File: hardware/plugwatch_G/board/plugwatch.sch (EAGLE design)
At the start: 176 parts, among them J1 DM3AT-SF-PEJM5, J2 SCREW_TERMNIAL_1, J3 SCREW_TERMNIAL_1, J4 TC2030-JLINK-L, Q1 NX3008PBK, Q2 MOSFET-NCHANNELSMD, U1 AB1815-T3, U10 STM32L432KC, U11 SIP32510, U12 SIP32510, U13 ADA4096-4ACPZ-R7, U14 SIP32510, U15 REF2030AIDDCR, U16 TCA9406DCUR, U17 SN74LVC1G86DBVR, U18 SN74LVC1G86DBVR, U2 BGA725L6-ALT, U21 SN74LVC1G86DBVR, U22 SN74LVC1G86DBVR, U3 DS2401P+, U4 SAFFB1G56KB0F0A, U5 IRM-03-5V, U6 LIS2DH12, U7 MAX-M8, U8 MAX67XXMAX6749MAX67XX, U9 TPS79330DBVR, X1 ABS07-32.768KHZ-7-T, X2 ABS05-32.768KHZ-T

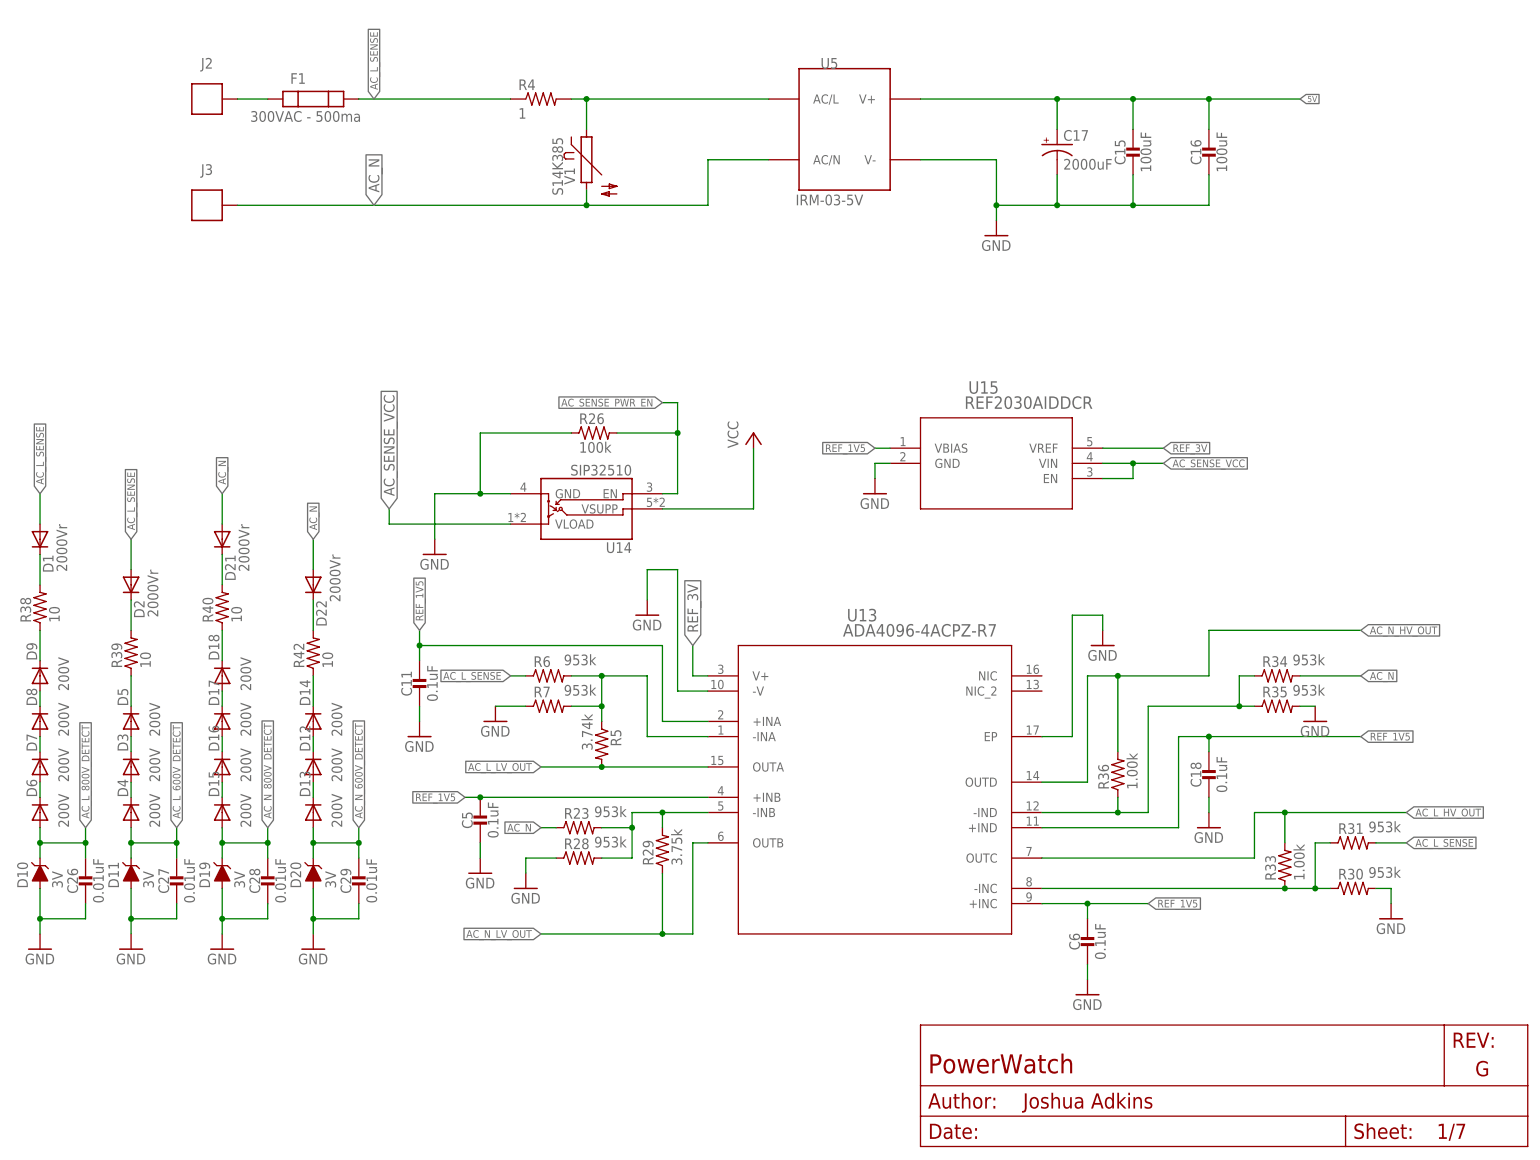
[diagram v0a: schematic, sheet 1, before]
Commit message: split the symbol up for the op amp so it's readable
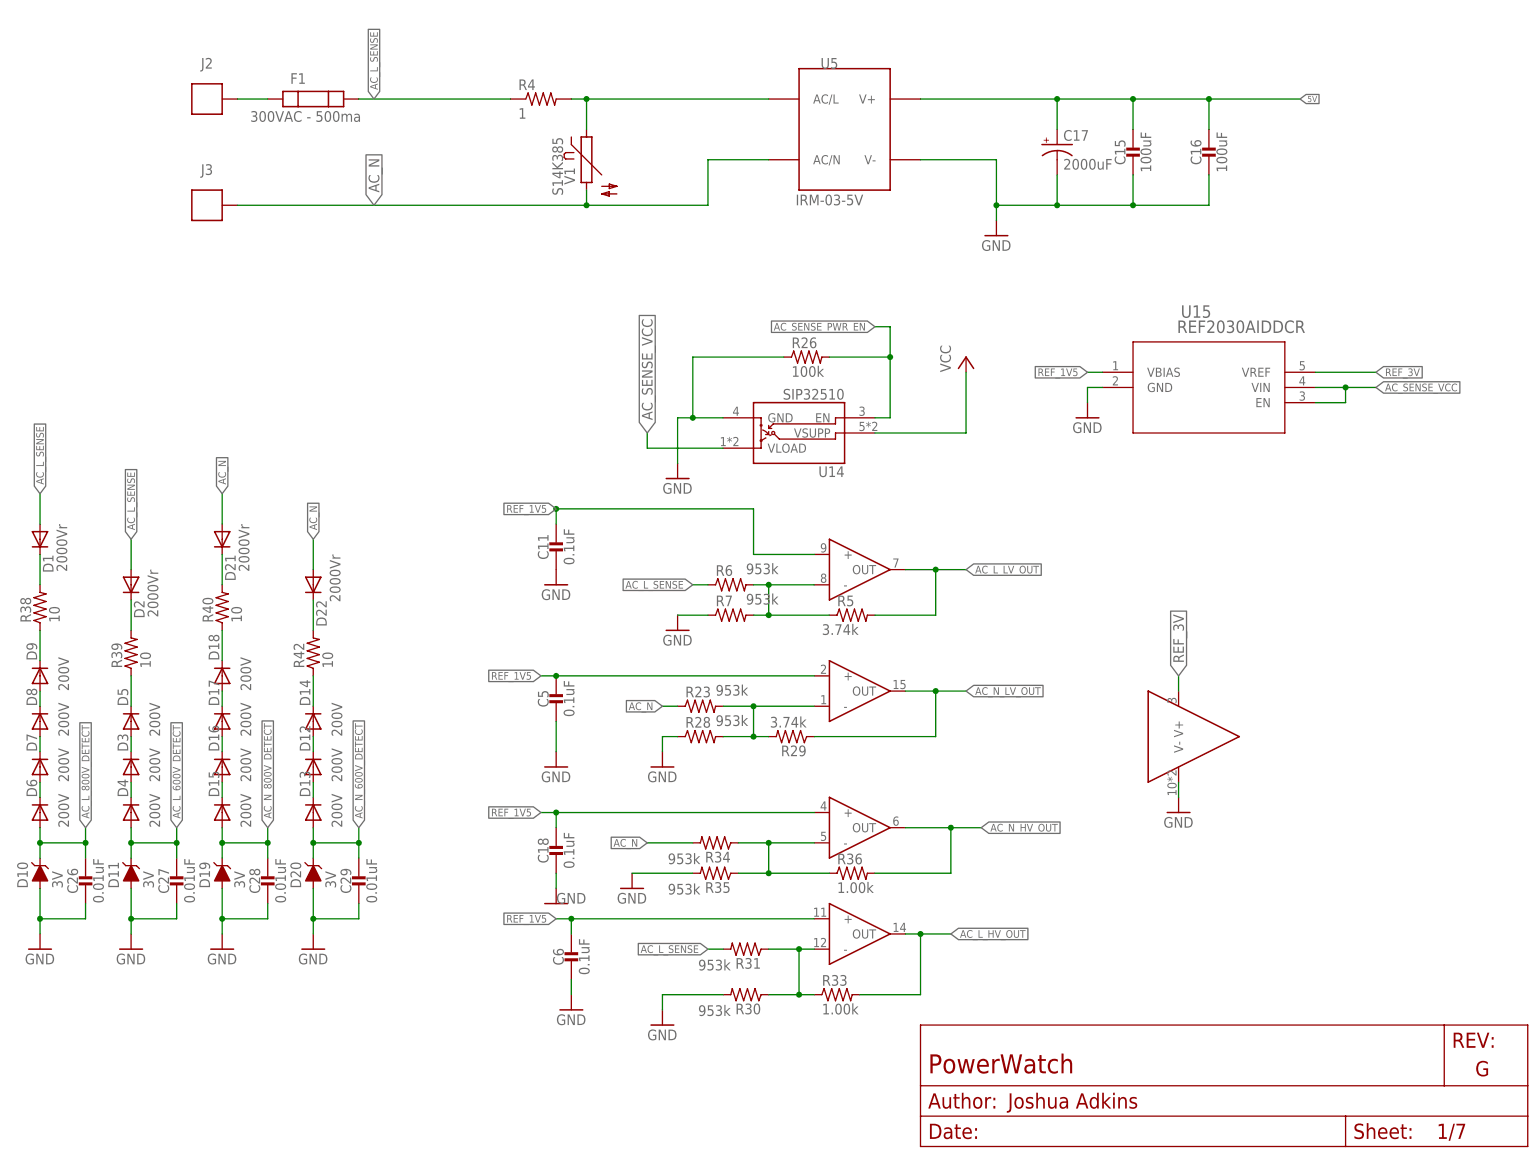
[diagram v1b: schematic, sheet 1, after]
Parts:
- R29: value 3.75k -> 3.74k
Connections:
- net AC_L_HV_OUT: now also U13D.OUT; no longer U13.OUTC
- net AC_L_LV_OUT: now also U13C.OUT; no longer U13.OUTA
- net AC_N_HV_OUT: now also U13B.OUT; no longer U13.OUTD
- net AC_N_LV_OUT: now also U13A.OUT; no longer U13.OUTB
- net GND: now also U13SUPPLY.V-; no longer U13.-V, U13.EP
- net N$3: now also U13A.-; no longer U13.-INB
- net N$4: now also U13C.-; no longer U13.-INA
- net N$6: now also U13D.-; no longer U13.-INC
- net N$8: now also U13B.-; no longer U13.-IND
- net REF_1V5: now also U13A.+, U13B.+, U13C.+, U13D.+; no longer U13.+INA, U13.+INB, U13.+INC, U13.+IND
- net REF_3V: now also U13SUPPLY.V+; no longer U13.V+
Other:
- moved on the sheet: C11, C18, C5, C6, R23, R26, R28, R29, R30, R31, R33, R34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

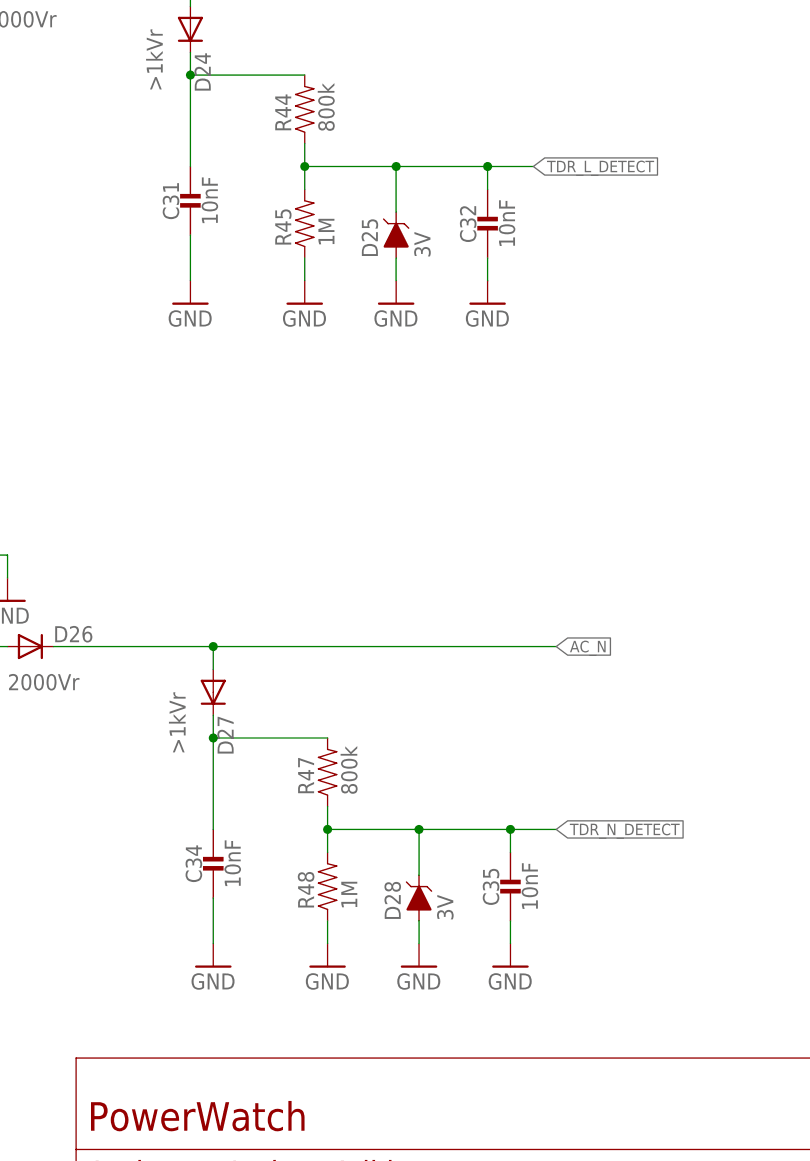
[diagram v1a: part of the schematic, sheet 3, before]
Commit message: add new plugwatch stuff
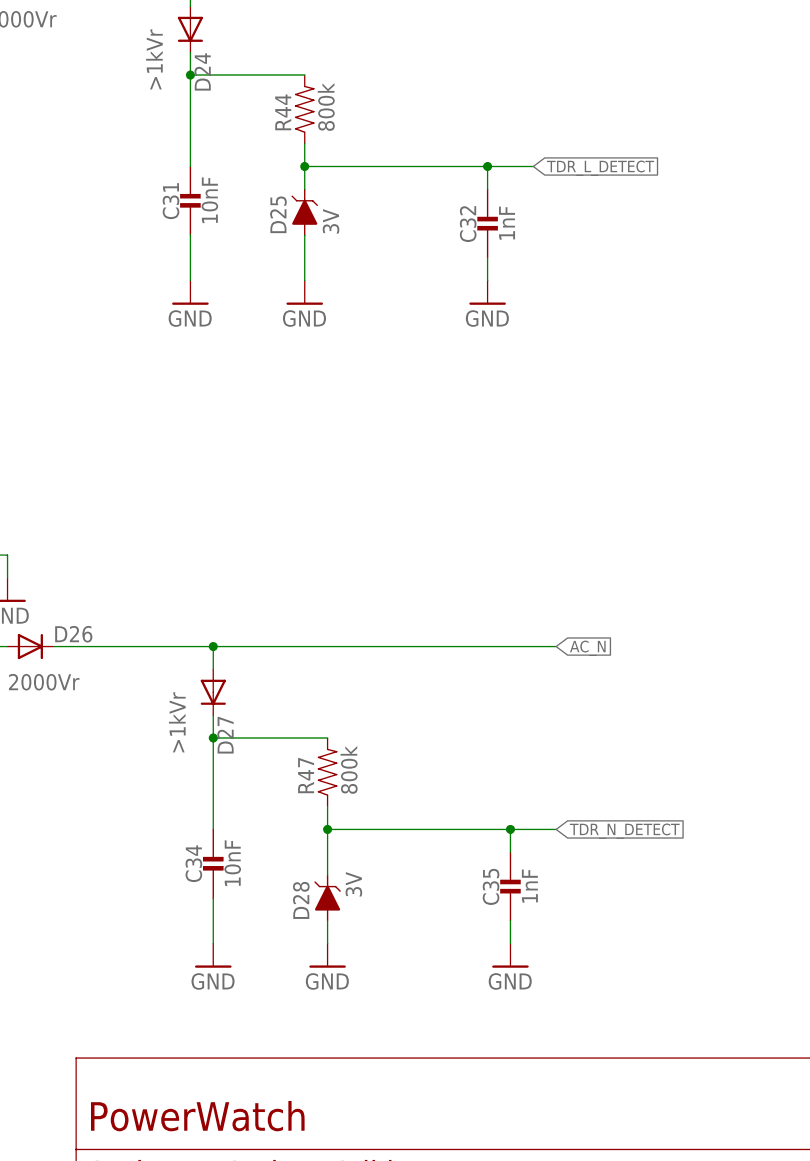
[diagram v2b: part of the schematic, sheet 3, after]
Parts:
- removed R45, R48: 1M, passives:RESISTOR0402_RES
- C32, C35: value 10nF -> 1nF
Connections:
- net GND: no longer R45.1, R48.1
- net TDR_L_DETECT: no longer R45.2
- net TDR_N_DETECT: no longer R48.2
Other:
- moved on the sheet: D25, D28
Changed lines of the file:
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@@
 <attribute name="MPN" value="CRCW0402100KFKED"/>
 </part>
-<part name="R45" library="passives" deviceset="RESISTOR" device="0402_RES" value="1M">
-<attribute name="DESCRIPTION" value="RES SMD 100K OHM 1% 1/16W 0402"/>
-<attribute name="DIGIKEY" value="541-100KLCT-ND"/>
-<attribute name="MANUFACTURER" value="Vishay Dale"/>
-<attribute name="MPN" value="CRCW0402100KFKED"/>
-</part>
-<part name="SUPPLY30" library="umich" deviceset="GND" device=""/>
-<part name="C32" library="passives" deviceset="CAPACITOR" device="0402_CAP" value="10nF">
+<part name="C32" library="passives" deviceset="CAPACITOR" device="0402_CAP" value="1nF">
 <attribute name="DESCRIPTION" value="CAP CER 0.1UF 10V X5R 0402"/>
 <attribute name="DIGIKEY" value="311-1336-1-ND"/>
@@
 <attribute name="MPN" value="CRCW0402100KFKED"/>
 </part>
-<part name="R48" library="passives" deviceset="RESISTOR" device="0402_RES" value="1M">
-<attribute name="DESCRIPTION" value="RES SMD 100K OHM 1% 1/16W 0402"/>
-<attribute name="DIGIKEY" value="541-100KLCT-ND"/>
-<attribute name="MANUFACTURER" value="Vishay Dale"/>
-<attribute name="MPN" value="CRCW0402100KFKED"/>
-</part>
-<part name="SUPPLY39" library="umich" deviceset="GND" device=""/>
-<part name="C35" library="passives" deviceset="CAPACITOR" device="0402_CAP" value="10nF">
+<part name="C35" library="passives" deviceset="CAPACITOR" device="0402_CAP" value="1nF">
 <attribute name="DESCRIPTION" value="CAP CER 0.1UF 10V X5R 0402"/>
 <attribute name="DIGIKEY" value="311-1336-1-ND"/>
@@
 <attribute name="VALUE" x="181.102" y="123.19" size="1.778" layer="96" rot="R90"/>
 </instance>
-<instance part="R45" gate="G$1" x="177.8" y="114.3" smashed="yes" rot="R90">
-<attribute name="DIGIKEY" x="177.8" y="114.3" size="1.27" layer="96" font="vector" rot="R90" display="off"/>
-<attribute name="NAME" x="176.3014" y="110.49" size="1.778" layer="95" rot="R90"/>
-<attribute name="VALUE" x="181.102" y="110.49" size="1.778" layer="96" rot="R90"/>
-</instance>
-<instance part="SUPPLY30" gate="1" x="177.8" y="104.14" smashed="yes">
-<attribute name="VALUE" x="175.26" y="101.6" size="1.778" layer="96"/>
-</instance>
 <instance part="C32" gate="G$1" x="198.12" y="114.3" smashed="yes">
 <attribute name="DIGIKEY" x="198.12" y="114.3" size="1.016" layer="96" rot="R270" align="bottom-center" display="off"/>
@@
 <attribute name="VALUE" x="195.58" y="101.6" size="1.778" layer="96"/>
 </instance>
-<instance part="D25" gate="G$1" x="187.96" y="111.76" smashed="yes" rot="R90">
-<attribute name="NAME" x="185.928" y="109.22" size="1.778" layer="95" font="vector" rot="R90"/>
-<attribute name="VALUE" x="189.992" y="109.22" size="1.778" layer="96" font="vector" rot="R90" align="top-left"/>
-</instance>
-<instance part="SUPPLY33" gate="1" x="187.96" y="104.14" smashed="yes">
-<attribute name="VALUE" x="185.42" y="101.6" size="1.778" layer="96"/>
+<instance part="D25" gate="G$1" x="177.8" y="114.3" smashed="yes" rot="R90">
+<attribute name="NAME" x="175.768" y="111.76" size="1.778" layer="95" font="vector" rot="R90"/>
+<attribute name="VALUE" x="179.832" y="111.76" size="1.778" layer="96" font="vector" rot="R90" align="top-left"/>
+</instance>
+<instance part="SUPPLY33" gate="1" x="177.8" y="104.14" smashed="yes">
+<attribute name="VALUE" x="175.26" y="101.6" size="1.778" layer="96"/>
 </instance>
 <instance part="U17" gate="A" x="30.48" y="68.58" smashed="yes" rot="MR180">
@@
 <attribute name="VALUE" x="183.642" y="49.53" size="1.778" layer="96" rot="R90"/>
 </instance>
-<instance part="R48" gate="G$1" x="180.34" y="40.64" smashed="yes" rot="R90">
-<attribute name="DIGIKEY" x="180.34" y="40.64" size="1.27" layer="96" font="vector" rot="R90" display="off"/>
-<attribute name="NAME" x="178.8414" y="36.83" size="1.778" layer="95" rot="R90"/>
-<attribute name="VALUE" x="183.642" y="36.83" size="1.778" layer="96" rot="R90"/>
-</instance>
-<instance part="SUPPLY39" gate="1" x="180.34" y="30.48" smashed="yes">
-<attribute name="VALUE" x="177.8" y="27.94" size="1.778" layer="96"/>
-</instance>
 <instance part="C35" gate="G$1" x="200.66" y="40.64" smashed="yes">
 <attribute name="DIGIKEY" x="200.66" y="40.64" size="1.016" layer="96" rot="R270" align="bottom-center" display="off"/>
@@
 <attribute name="VALUE" x="198.12" y="27.94" size="1.778" layer="96"/>
 </instance>
-<instance part="D28" gate="G$1" x="190.5" y="38.1" smashed="yes" rot="R90">
-<attribute name="NAME" x="188.468" y="35.56" size="1.778" layer="95" font="vector" rot="R90"/>
-<attribute name="VALUE" x="192.532" y="35.56" size="1.778" layer="96" font="vector" rot="R90" align="top-left"/>
-</instance>
-<instance part="SUPPLY41" gate="1" x="190.5" y="30.48" smashed="yes">
-<attribute name="VALUE" x="187.96" y="27.94" size="1.778" layer="96"/>
+<instance part="D28" gate="G$1" x="180.34" y="38.1" smashed="yes" rot="R90">
+<attribute name="NAME" x="178.308" y="35.56" size="1.778" layer="95" font="vector" rot="R90"/>
+<attribute name="VALUE" x="182.372" y="38.1" size="1.778" layer="96" font="vector" rot="R90" align="top-left"/>
+</instance>
+<instance part="SUPPLY41" gate="1" x="180.34" y="30.48" smashed="yes">
+<attribute name="VALUE" x="177.8" y="27.94" size="1.778" layer="96"/>
 </instance>
 </instances>
@@
 </segment>
 <segment>
-<pinref part="SUPPLY30" gate="1" pin="GND"/>
-<pinref part="R45" gate="G$1" pin="1"/>
-<wire x1="177.8" y1="106.68" x2="177.8" y2="109.22" width="0.1524" layer="91"/>
-</segment>
-<segment>
 <pinref part="D25" gate="G$1" pin="A"/>
-<wire x1="187.96" y1="109.22" x2="187.96" y2="106.68" width="0.1524" layer="91"/>
+<wire x1="177.8" y1="111.76" x2="177.8" y2="106.68" width="0.1524" layer="91"/>
 <pinref part="SUPPLY33" gate="1" pin="GND"/>
 </segment>
@@
 </segment>
 <segment>
-<pinref part="SUPPLY39" gate="1" pin="GND"/>
-<pinref part="R48" gate="G$1" pin="1"/>
-<wire x1="180.34" y1="33.02" x2="180.34" y2="35.56" width="0.1524" layer="91"/>
-</segment>
-<segment>
 <pinref part="D28" gate="G$1" pin="A"/>
-<wire x1="190.5" y1="35.56" x2="190.5" y2="33.02" width="0.1524" layer="91"/>
+<wire x1="180.34" y1="35.56" x2="180.34" y2="33.02" width="0.1524" layer="91"/>
 <pinref part="SUPPLY41" gate="1" pin="GND"/>
 </segment>
@@
 <segment>
 <pinref part="D25" gate="G$1" pin="C"/>
-<wire x1="187.96" y1="114.3" x2="187.96" y2="119.38" width="0.1524" layer="91"/>
-<pinref part="R45" gate="G$1" pin="2"/>
+<wire x1="177.8" y1="116.84" x2="177.8" y2="119.38" width="0.1524" layer="91"/>
 <pinref part="R44" gate="G$1" pin="1"/>
-<wire x1="177.8" y1="116.84" x2="177.8" y2="119.38" width="0.1524" layer="91"/>
 <wire x1="177.8" y1="119.38" x2="177.8" y2="121.92" width="0.1524" layer="91"/>
-<wire x1="187.96" y1="119.38" x2="177.8" y2="119.38" width="0.1524" layer="91"/>
-<junction x="177.8" y="119.38"/>
 <pinref part="C32" gate="G$1" pin="1"/>
 <wire x1="198.12" y1="116.84" x2="198.12" y2="119.38" width="0.1524" layer="91"/>
-<wire x1="198.12" y1="119.38" x2="187.96" y2="119.38" width="0.1524" layer="91"/>
-<junction x="187.96" y="119.38"/>
+<wire x1="198.12" y1="119.38" x2="177.8" y2="119.38" width="0.1524" layer="91"/>
+<junction x="177.8" y="119.38"/>
 <wire x1="198.12" y1="119.38" x2="203.2" y2="119.38" width="0.1524" layer="91"/>
 <junction x="198.12" y="119.38"/>
@@
 <segment>
 <pinref part="D28" gate="G$1" pin="C"/>
-<wire x1="190.5" y1="40.64" x2="190.5" y2="45.72" width="0.1524" layer="91"/>
-<pinref part="R48" gate="G$1" pin="2"/>
+<wire x1="180.34" y1="40.64" x2="180.34" y2="45.72" width="0.1524" layer="91"/>
 <pinref part="R47" gate="G$1" pin="1"/>
-<wire x1="180.34" y1="43.18" x2="180.34" y2="45.72" width="0.1524" layer="91"/>
 <wire x1="180.34" y1="45.72" x2="180.34" y2="48.26" width="0.1524" layer="91"/>
-<wire x1="190.5" y1="45.72" x2="180.34" y2="45.72" width="0.1524" layer="91"/>
-<junction x="180.34" y="45.72"/>
 <pinref part="C35" gate="G$1" pin="1"/>
 <wire x1="200.66" y1="43.18" x2="200.66" y2="45.72" width="0.1524" layer="91"/>
-<wire x1="200.66" y1="45.72" x2="190.5" y2="45.72" width="0.1524" layer="91"/>
-<junction x="190.5" y="45.72"/>
+<wire x1="200.66" y1="45.72" x2="180.34" y2="45.72" width="0.1524" layer="91"/>
+<junction x="180.34" y="45.72"/>
 <wire x1="200.66" y1="45.72" x2="205.74" y2="45.72" width="0.1524" layer="91"/>
 <junction x="200.66" y="45.72"/>
